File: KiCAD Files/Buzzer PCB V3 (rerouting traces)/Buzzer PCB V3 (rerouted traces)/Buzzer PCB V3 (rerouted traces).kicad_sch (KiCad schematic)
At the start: 28 parts, among them J1 2600mAh LiPo JST-PH bottom, J10 SparkFun Thing Plus ESP32 WRO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, J11 M16968 OLED + Rotary Knob, J5 HGLRC M100 Mini GPS, J6 BMP581/BMP5xx top pads, J7 SHT41 top pads, Q1 S8050, Q2 S8050, Q3 S8050, SW1 SS12F44G3 power switch, U1 TP4057 USB-C charger, U2 Comidox 5V Booster

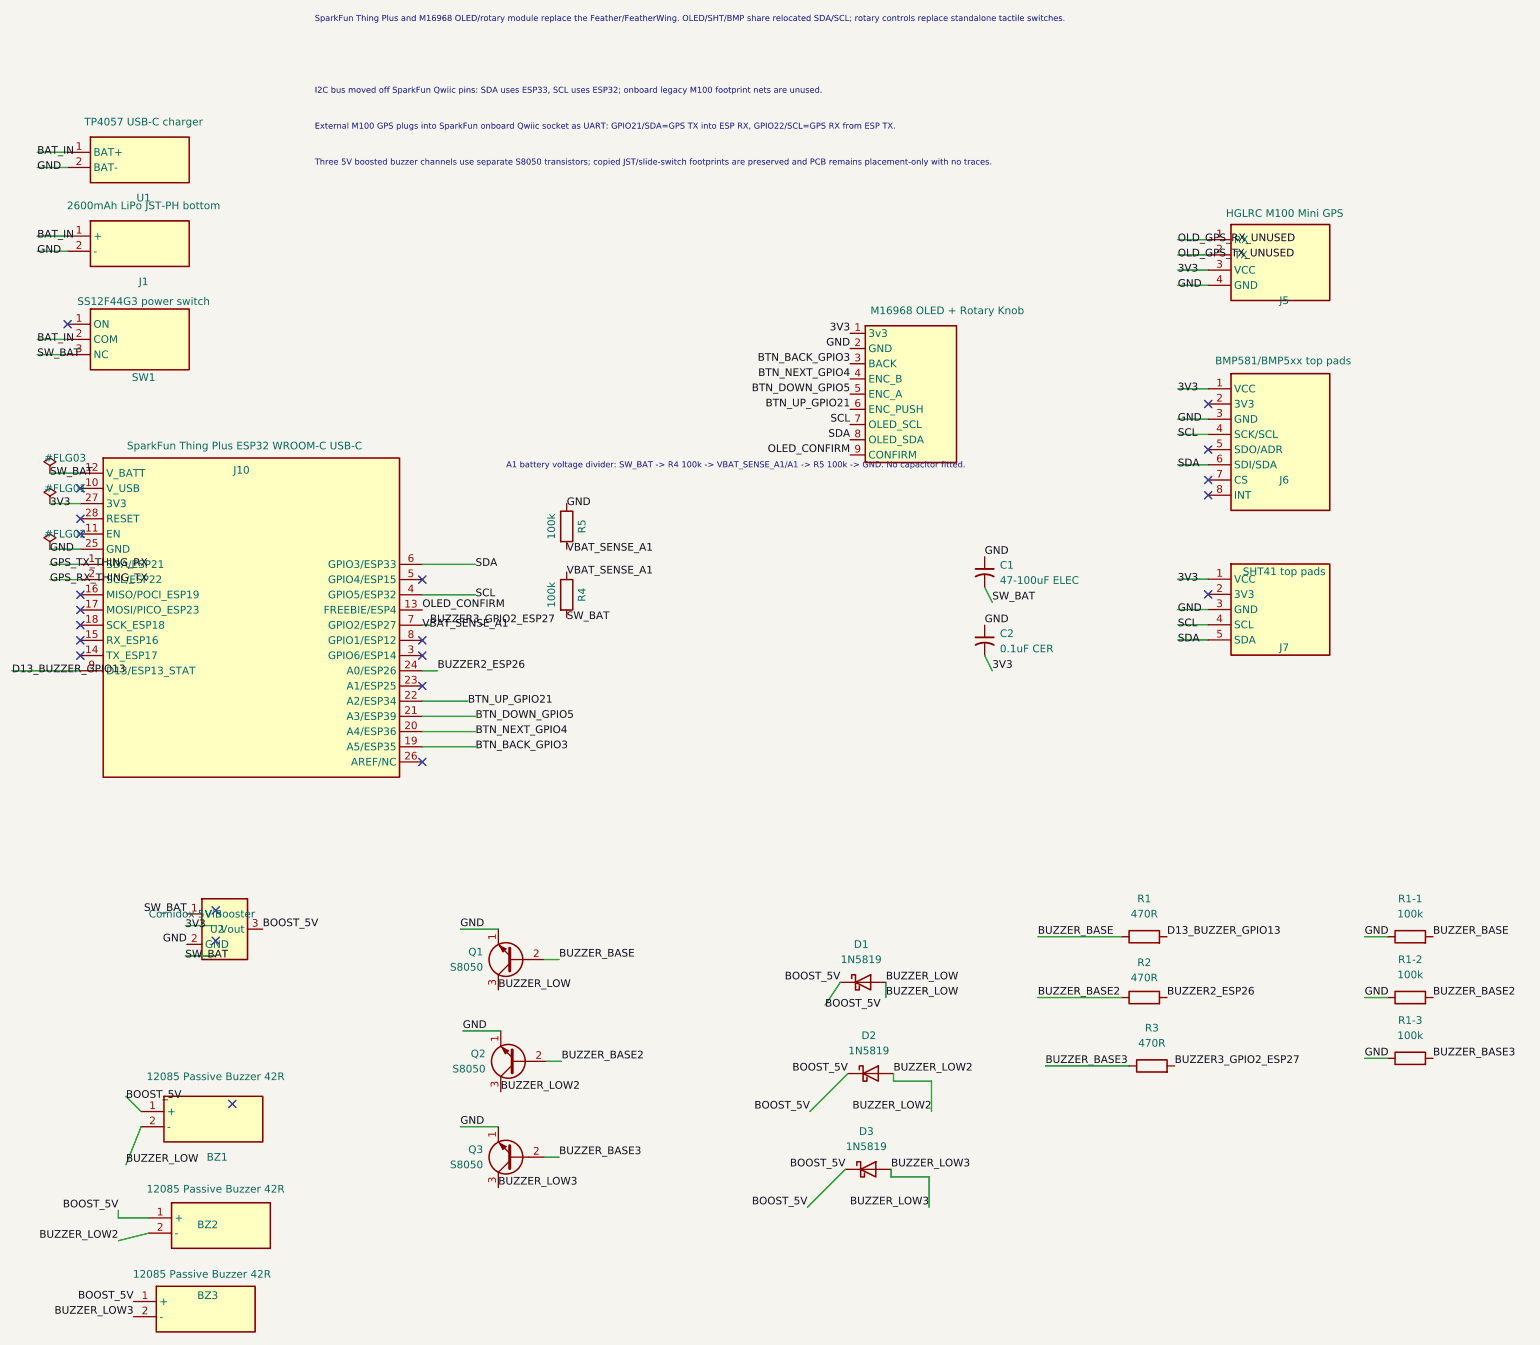
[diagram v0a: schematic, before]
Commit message: FInal Sparkfun Version
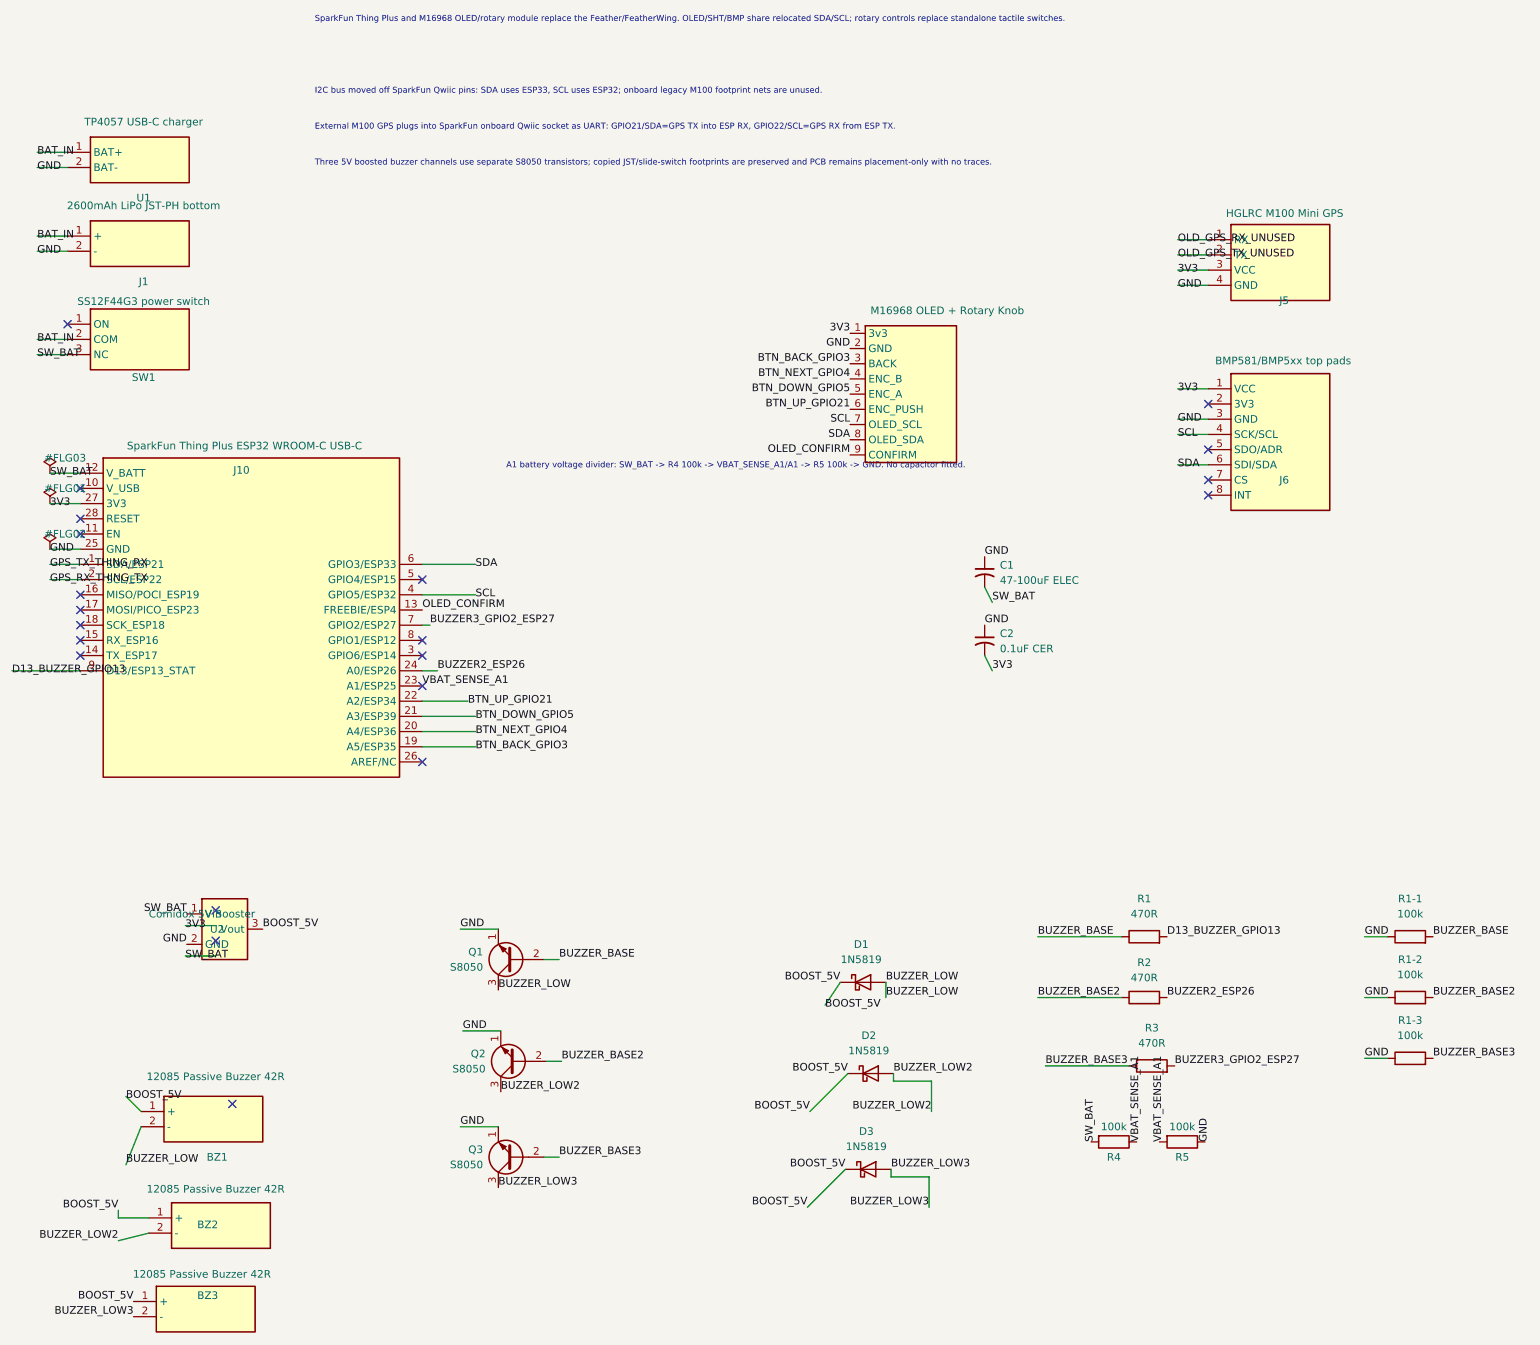
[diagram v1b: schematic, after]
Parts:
- removed J7: SHT41 top pads, Vario_Buzzer_V2:Adafruit_SHT41_Breakout_Top, symbol Vario_Buzzer_V2:SHT41_5
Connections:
- net BUZZER3_GPIO2_ESP27: no longer R4.1, R5.2
- net VBAT_SENSE_A1: now reaches J10.23 (A1/ESP25)
- net VBAT_SENSE_A1: now also R4.1, R5.2
- no-connect marks 22 -> 21
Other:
- moved on the sheet: R4, R5
